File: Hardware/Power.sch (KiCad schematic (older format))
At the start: 32 parts, among them J6 Barrel_Jack_MountingPin, U10 LM2734Y, U8 LM2734Y, U9 LM2611xMF

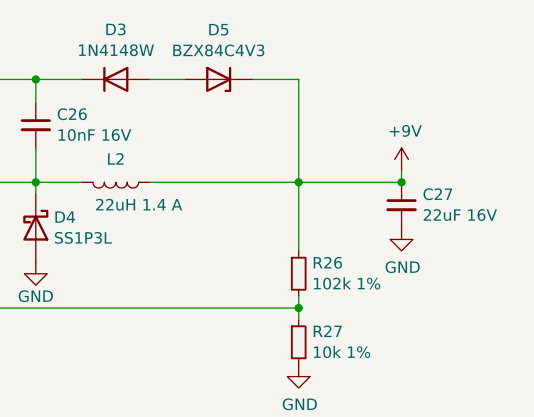
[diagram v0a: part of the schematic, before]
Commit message: ERC check on the schematics
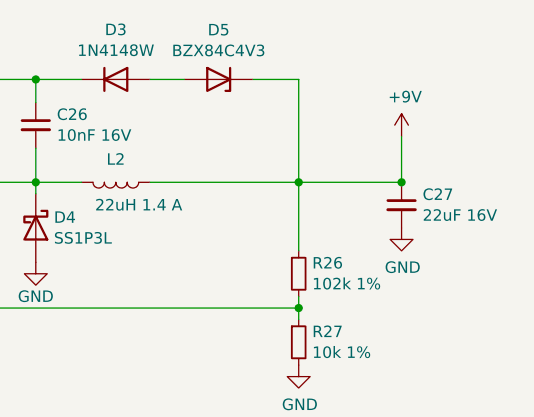
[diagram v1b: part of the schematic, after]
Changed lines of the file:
@@
 L power:+9V #PWR021
 U 1 1 5D1829E8
-P 10200 2050
-F 0 "#PWR021" H 10200 1900 50  0001 C CNN
-F 1 "+9V" H 10215 2223 50  0000 C CNN
-F 2 "" H 10200 2050 50  0001 C CNN
-F 3 "" H 10200 2050 50  0001 C CNN
-	1    10200 2050
+P 10200 1900
+F 0 "#PWR021" H 10200 1750 50  0001 C CNN
+F 1 "+9V" H 10215 2073 50  0000 C CNN
+F 2 "" H 10200 1900 50  0001 C CNN
+F 3 "" H 10200 1900 50  0001 C CNN
+	1    10200 1900
 	1    0    0    -1
 $EndComp
@@
 $EndComp
 Wire Wire Line
-	10200 2050 10200 2100
+	10200 1900 10200 2100
 Wire Wire Line
 	10200 2100 9750 2100
